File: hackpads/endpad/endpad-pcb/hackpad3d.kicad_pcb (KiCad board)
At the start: 2 copper layers, 98.7 x 80.7 mm, 23 parts, among them SW1 SW_Push, SW10 SW_Push, SW11 SW_Push, SW12 SW_Push, SW13 SW_Push, SW14 SW_Push, SW15 SW_Push, SW16 SW_Push, SW2 SW_Push, SW3 SW_Push, SW4 SW_Push, SW5 SW_Push, SW6 RotaryEncoder_Switch, SW7 SW_Push, SW8 SW_Push, SW9 SW_Push, U1 XIAO-RP2040-DIP, U2 MCP23017_SO

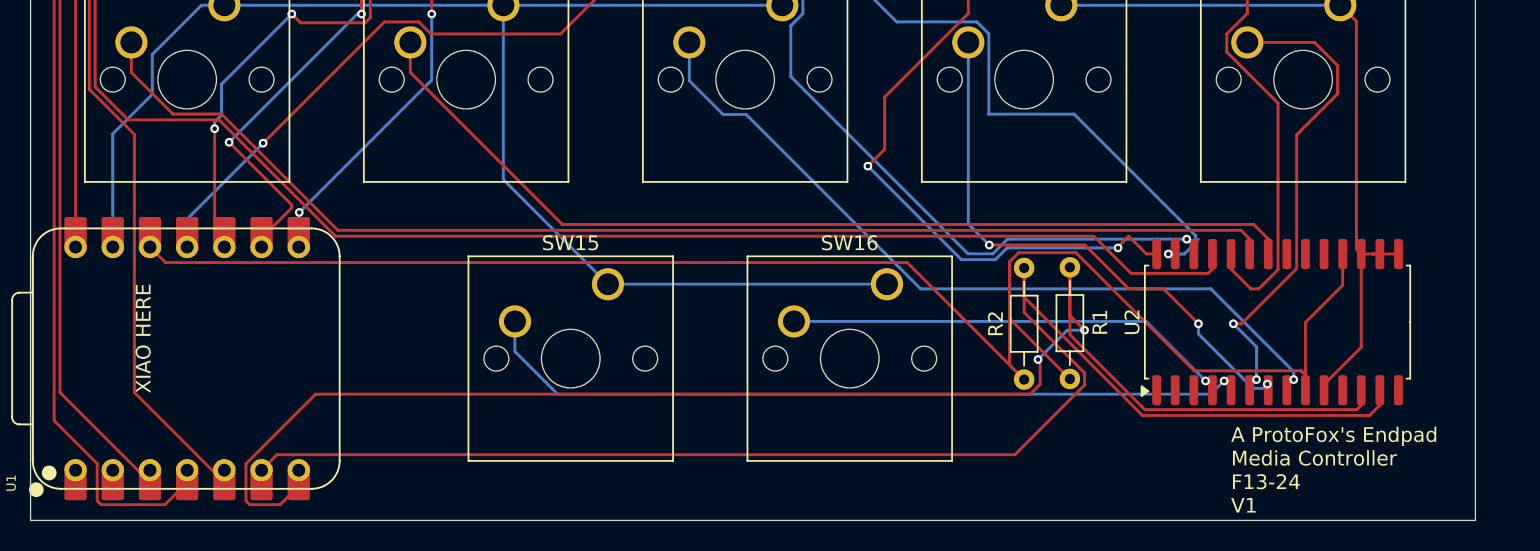
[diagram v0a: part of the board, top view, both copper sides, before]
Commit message: o
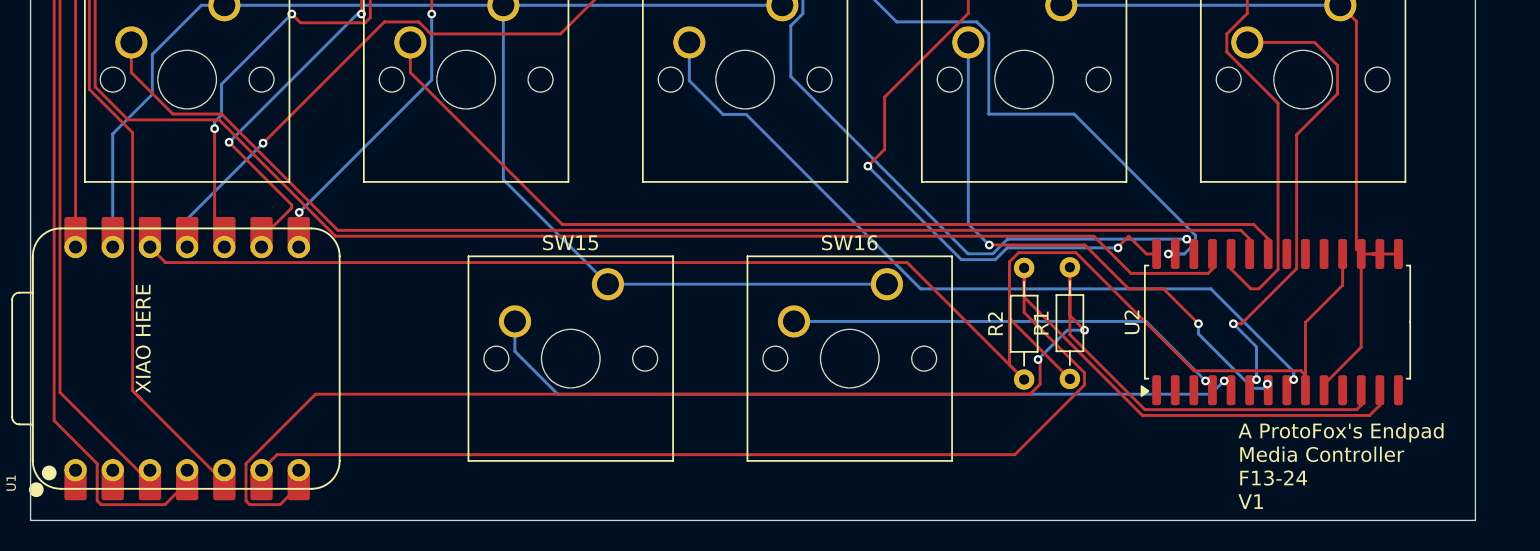
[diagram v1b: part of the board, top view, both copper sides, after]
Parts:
- G***: footprint LOGO -> 3D Models:LOGO
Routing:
- net Net-(U2-GPA5): track 77.5 -> 75.8 mm
- net Net-(U1-GPIO0/TX): track 102.5 -> 101.5 mm
- net Net-(U1-GPIO4/MISO): track 61.7 -> 60.7 mm
- net ENC-B: track 154.0 -> 153.2 mm
- net Net-(D1-DIN): track 126.8 -> 127.5 mm
- net Net-(U1-GPIO2/SCK): track 75.6 -> 75.0 mm
